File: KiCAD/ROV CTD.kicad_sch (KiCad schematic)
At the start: 43 parts, among them J1 Conn_Coaxial, J10 1Wire1, J11 1Wire2, J12 1Wire3, J13 Interface, J14 Interface, J15 Conn_01x07_Pin, J6 Main In, M1 EZO-EC, M2 MS5803-14BA, U2 ATtiny1614-Arduino, U3 AP63205WU, U6 MAX3072E

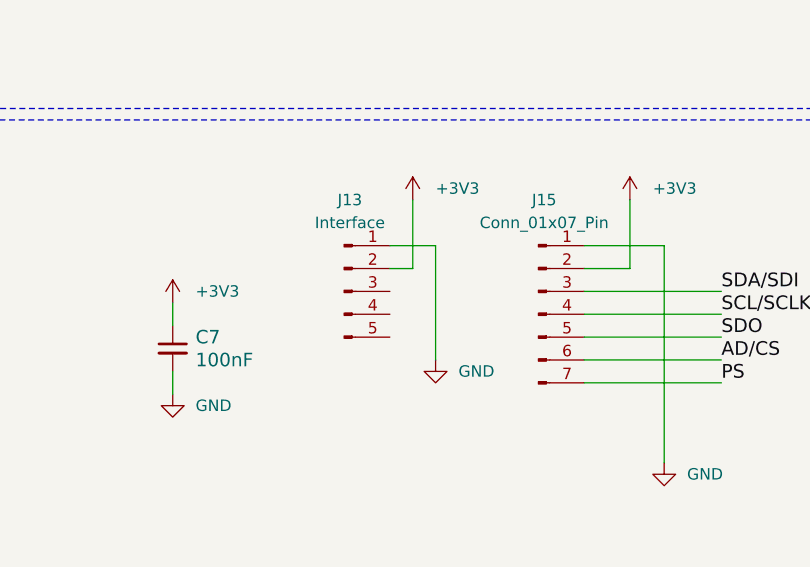
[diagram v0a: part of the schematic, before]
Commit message: .
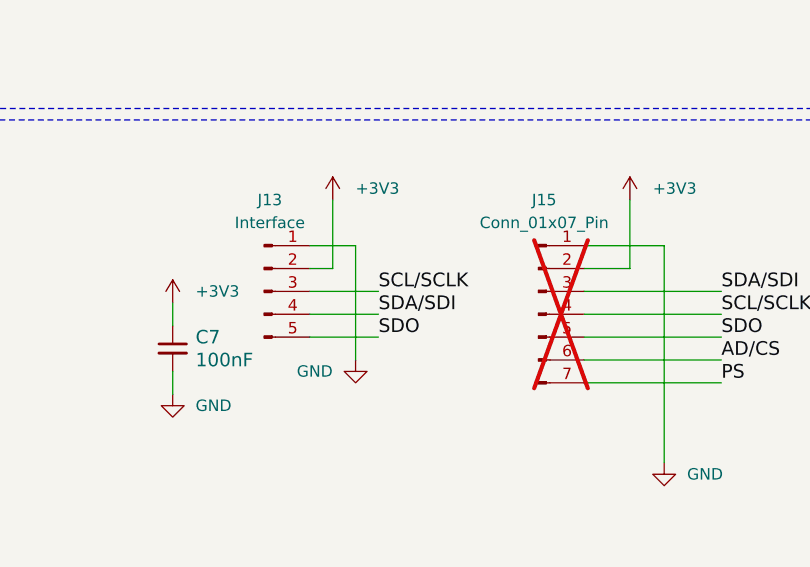
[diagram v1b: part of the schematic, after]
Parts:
- J15: now not fitted
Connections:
- net SCL/SCLK: now also J13.3 (Pin_3)
- net SDA/SDI: now also J13.4 (Pin_4)
- net SDO: now also J13.5 (Pin_5)
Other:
- moved on the sheet: J13
